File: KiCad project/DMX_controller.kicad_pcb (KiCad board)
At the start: 2 copper layers, 8 parts, among them J1 DMX_output, SW1 SW_Push_DPDT, U1 TTL_to_RS485_transceiver

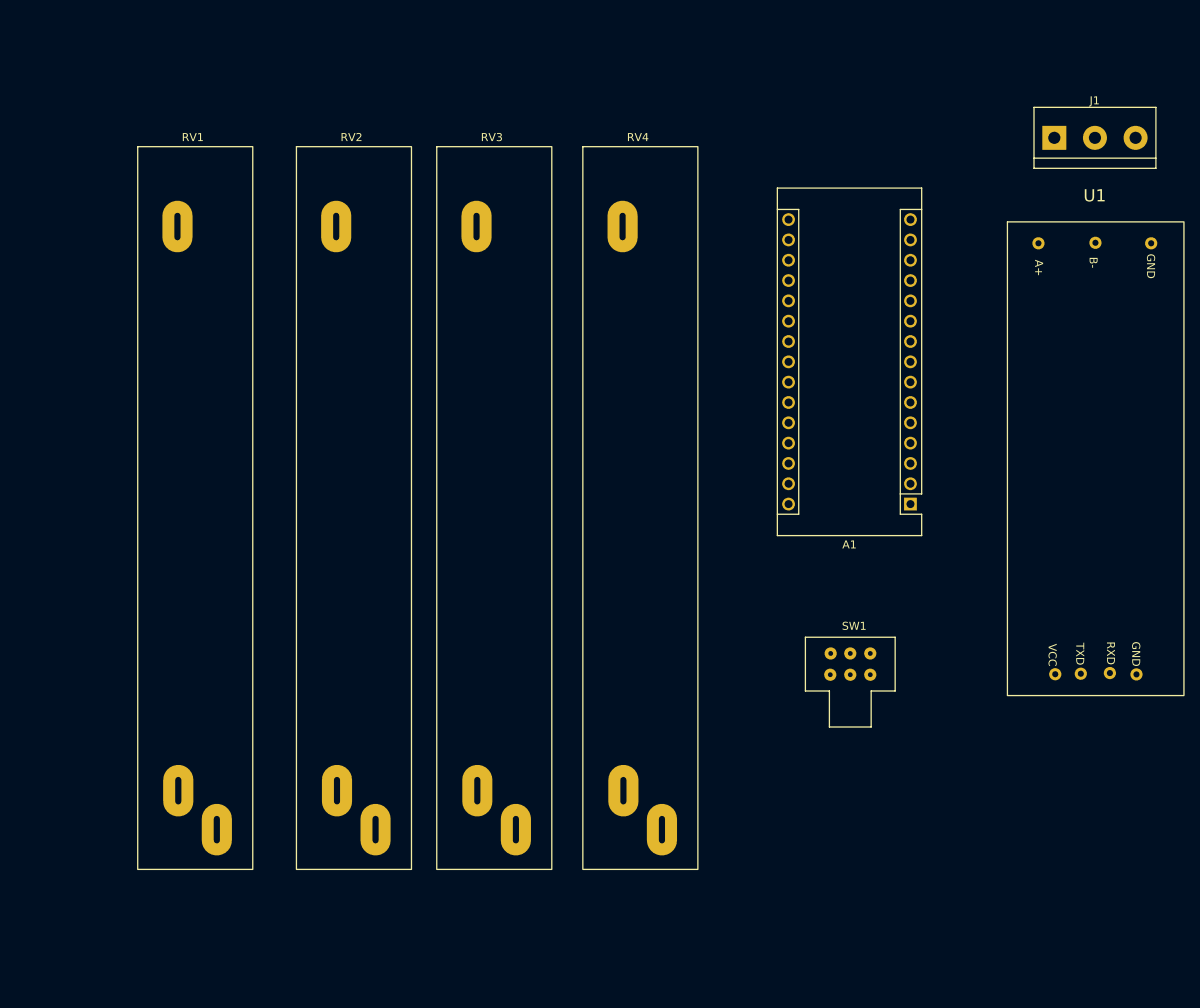
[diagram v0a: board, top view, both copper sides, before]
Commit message: Make a real PCB!
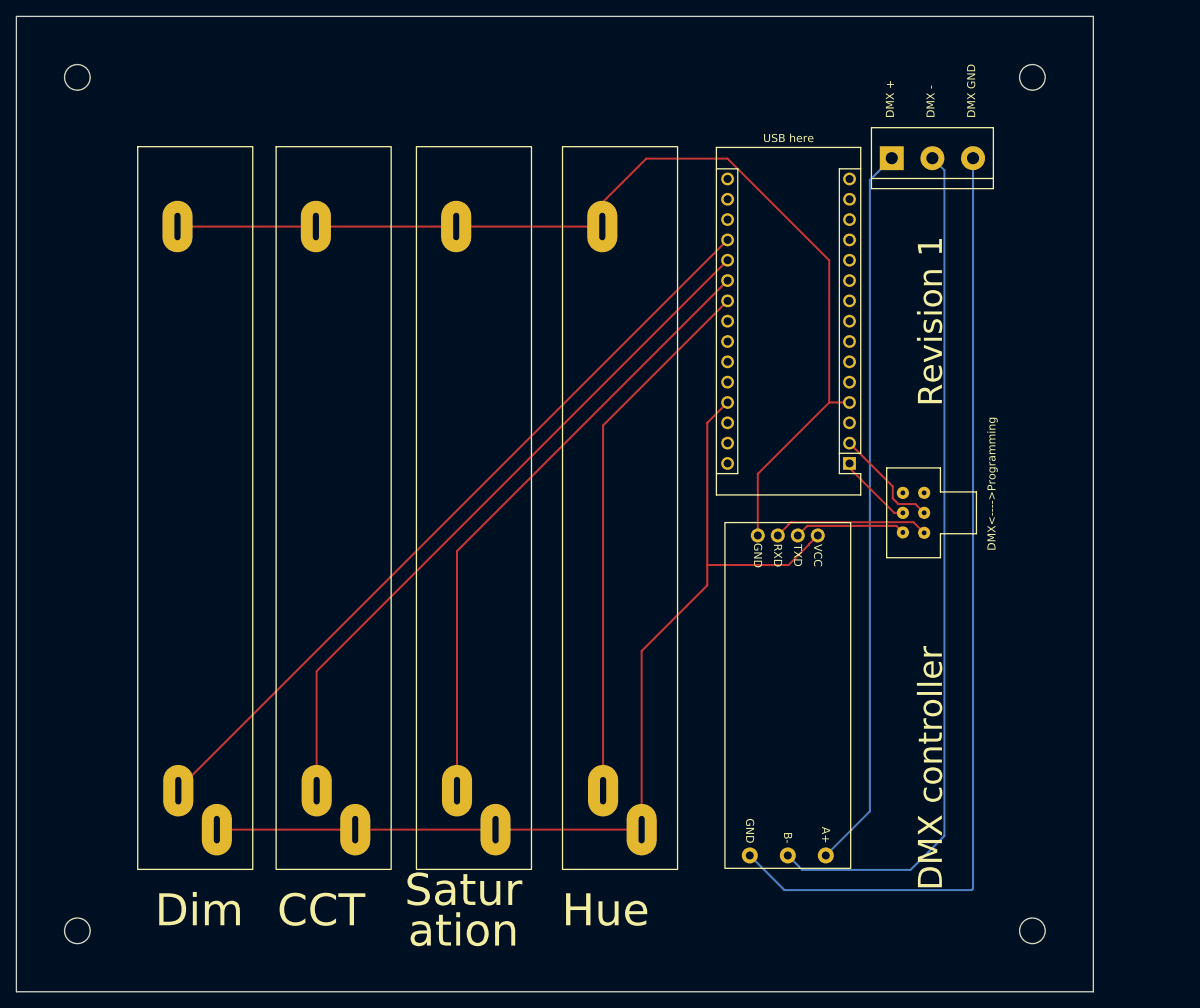
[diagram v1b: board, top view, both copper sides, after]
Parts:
- added REF**: MountingHole_3.2mm_M3, MountingHole:MountingHole_3.2mm_M3, F.Cu at (53.3, 43.2)
- added REF**: MountingHole_3.2mm_M3, MountingHole:MountingHole_3.2mm_M3, F.Cu at (172.7, 149.9)
- added REF**: MountingHole_3.2mm_M3, MountingHole:MountingHole_3.2mm_M3, F.Cu at (53.3, 149.9)
- added REF**: MountingHole_3.2mm_M3, MountingHole:MountingHole_3.2mm_M3, F.Cu at (172.7, 43.2)
- RV3: value slider_3_hue -> slider_3_saturation
- RV4: value slider_4_saturation -> slider_4_hue
- moved U1 31.4 mm to (149.9, 98.9), turned to -90 degrees
- moved J1 20.5 mm to (155.1, 53.3)
- moved SW1 14.4 mm to (154.6, 103.1), turned to 90 degrees
- moved A1 9.16 mm to (149.9, 91.4)
- moved RV3 2.54 mm to (96.2, 52.3)
- moved RV4 2.54 mm to (114.5, 52.3)
- moved RV2 2.54 mm to (78.7, 52.3)
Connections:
- net /5V renamed +5V
- A1 pad 29: /GND -> unconnected-(A1-Pad29)
- A1 pad 4: /GND -> GND
- RV1 pad 1: /GND -> GND
- RV2 pad 1: /GND -> GND
- RV3 pad 1: /GND -> GND
- RV4 pad 1: /GND -> GND
- U1 pad 4: /GND -> GND
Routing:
- net GND: track 0.00 -> 132.6 mm
- net +5V: track 0.00 -> 126.3 mm
- net Net-(J1-Pad3): track 0.00 -> 121.1 mm
- net Net-(J1-Pad2): track 0.00 -> 107.4 mm
- net /A0: track 0.00 -> 97.3 mm
- net Net-(J1-Pad1): track 0.00 -> 90.6 mm
- net /A1: track 0.00 -> 87.6 mm
- net /A2: track 0.00 -> 77.8 mm
- net /A3: track 0.00 -> 67.7 mm
- net Net-(SW1-Pad4): track 0.00 -> 19.5 mm
- net Net-(SW1-Pad1): track 0.00 -> 14.0 mm
- net /RX: track 0.00 -> 13.8 mm
- net /TX: track 0.00 -> 9.57 mm
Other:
- board outline added: 134.6 x 121.9 mm
- board text added: "CCT"
- board text added: "DMX +"
- board text added: "DMX -"
- board text added: "DMX GND"
- board text added: "DMX controller"
- board text added: "DMX<---->Programming"
- board text added: "Dim"
- board text added: "Hue"
- board text added: "Revision 1"
- board text added: "Satur"
- board text added: "USB here"
- board text added: "ation"
